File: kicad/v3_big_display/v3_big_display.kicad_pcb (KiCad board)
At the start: 2 copper layers, 33.9 x 42.5 mm, 8 parts, among them SW1 SW_Push, SW2 SW_Push, U1 nice_nano, U2 GY-BNO08X, U3 SSD1306_OLED_042

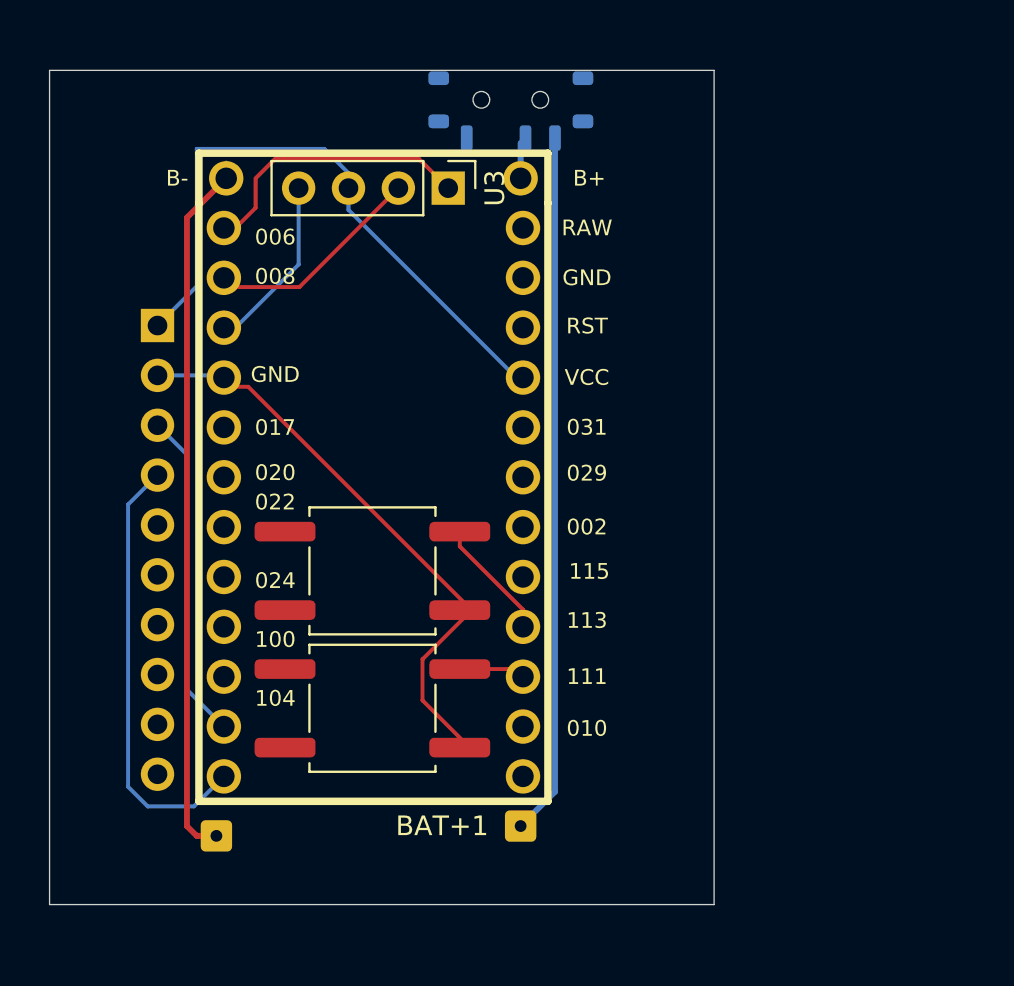
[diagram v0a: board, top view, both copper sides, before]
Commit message: kicad: tidy up
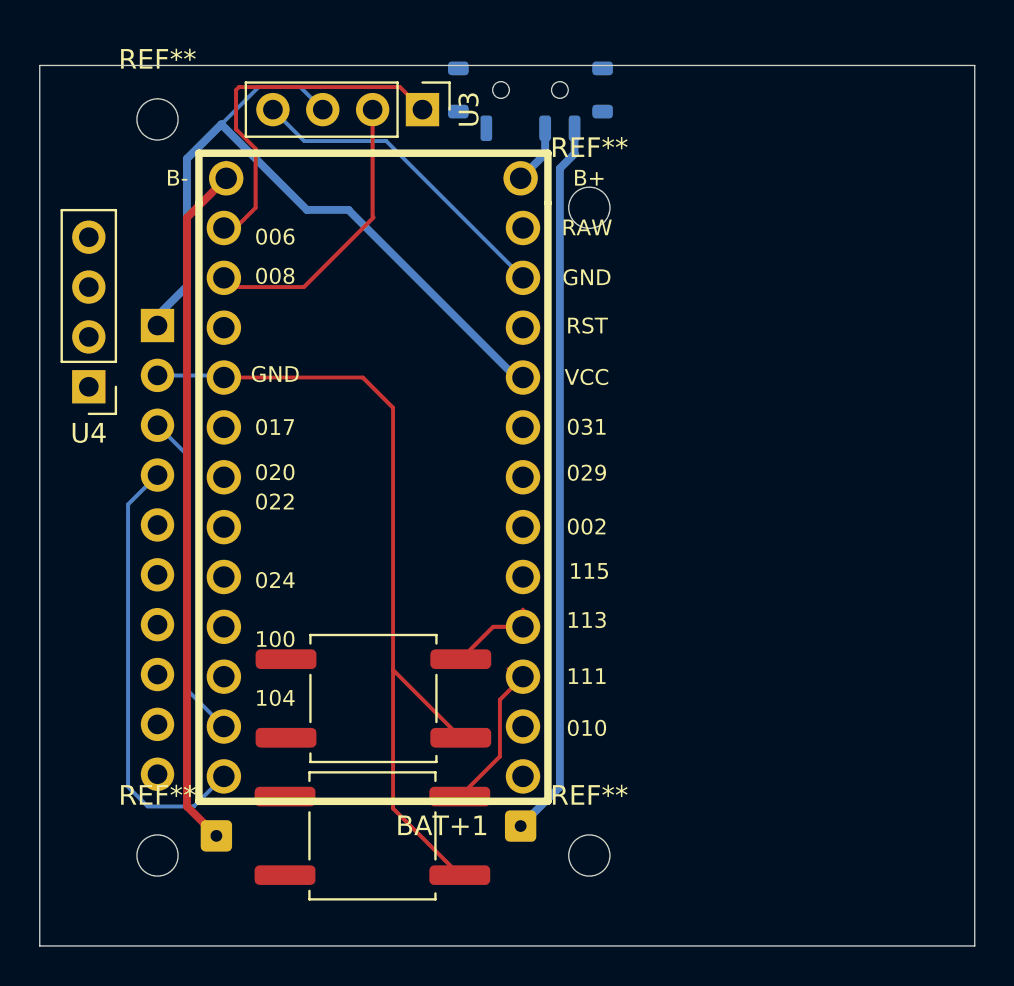
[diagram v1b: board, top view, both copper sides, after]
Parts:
- added REF**: MountingHole_2.1mm, MountingHole:MountingHole_2.1mm, F.Cu at (176.0, 49.0)
- added REF**: MountingHole_2.1mm, MountingHole:MountingHole_2.1mm, F.Cu at (198.0, 86.5)
- added REF**: MountingHole_2.1mm, MountingHole:MountingHole_2.1mm, F.Cu at (176.0, 86.5)
- added REF**: MountingHole_2.1mm, MountingHole:MountingHole_2.1mm, F.Cu at (198.0, 53.5)
- added U4: SSD1306_OLED_042, Connector_PinHeader_2.54mm:PinHeader_1x04_P2.54mm_Vertical, F.Cu at (172.5, 62.6)
- moved SW2 6.50 mm to (187.0, 78.5)
- moved SW1 6.50 mm to (186.9, 85.5)
- moved U3 4.21 mm to (189.5, 48.5)
- moved SW_POWER1 1.12 mm to (195.0, 47.5)
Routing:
- net GND: track 39.2 -> 59.5 mm
- net Net-(U1-VCC): track 32.7 -> 39.1 mm
- net Net-(U1-P1.11): track 4.60 -> 9.21 mm
- net Net-(U1-TX0/P0.06): track 14.5 -> 18.6 mm
- net Net-(U1-RX1/P0.08): track 10.9 -> 14.5 mm
- net Net-(U1-P1.13): track 6.18 -> 4.73 mm
- net Net-(BAT+1-Pin_1): track 35.3 -> 36.2 mm
- net Net-(BAT-1-Pin_1): track 37.5 -> 36.9 mm
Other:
- board size 33.9 x 42.5 mm -> 47.6 x 44.9 mm
